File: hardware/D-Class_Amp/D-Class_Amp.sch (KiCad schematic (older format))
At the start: 31 parts, among them J101 P_IN, J102 AudioJack2, U101 NCP1117-12_TO252, U102 MCP1799T-5002H_TT

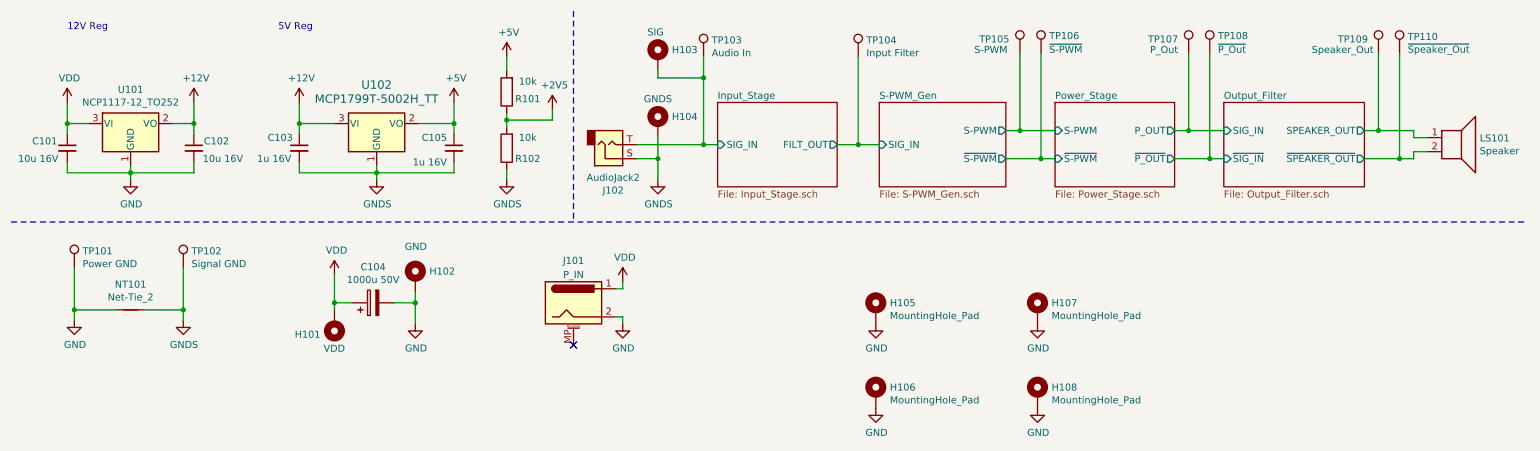
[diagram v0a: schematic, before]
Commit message: PCB done POG
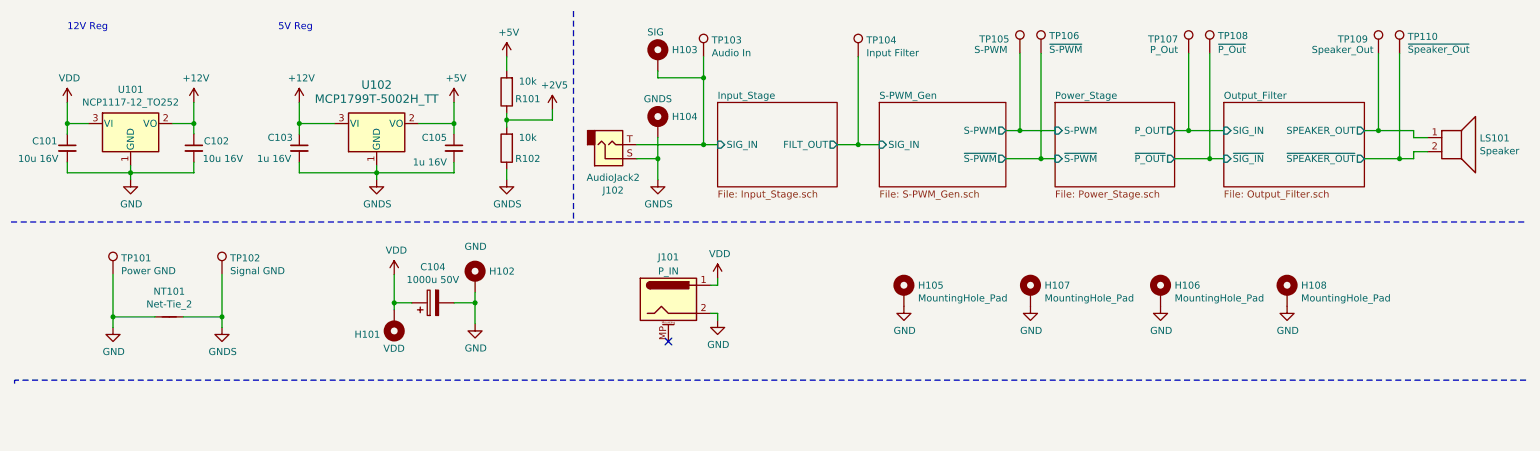
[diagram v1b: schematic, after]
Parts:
- J102: DigiKey Price (none) -> 2.27; Part Number (none) -> MJ-63022A
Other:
- moved on the sheet: C104, H101, H102, H105, H106, H107, H108, J101, NT101, TP101, TP102
